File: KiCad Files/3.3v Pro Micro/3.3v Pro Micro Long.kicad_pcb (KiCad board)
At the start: 2 copper layers, 35.7 x 48.3 mm, 5 parts, among them U2 ProMicro, U3 BOB-12009

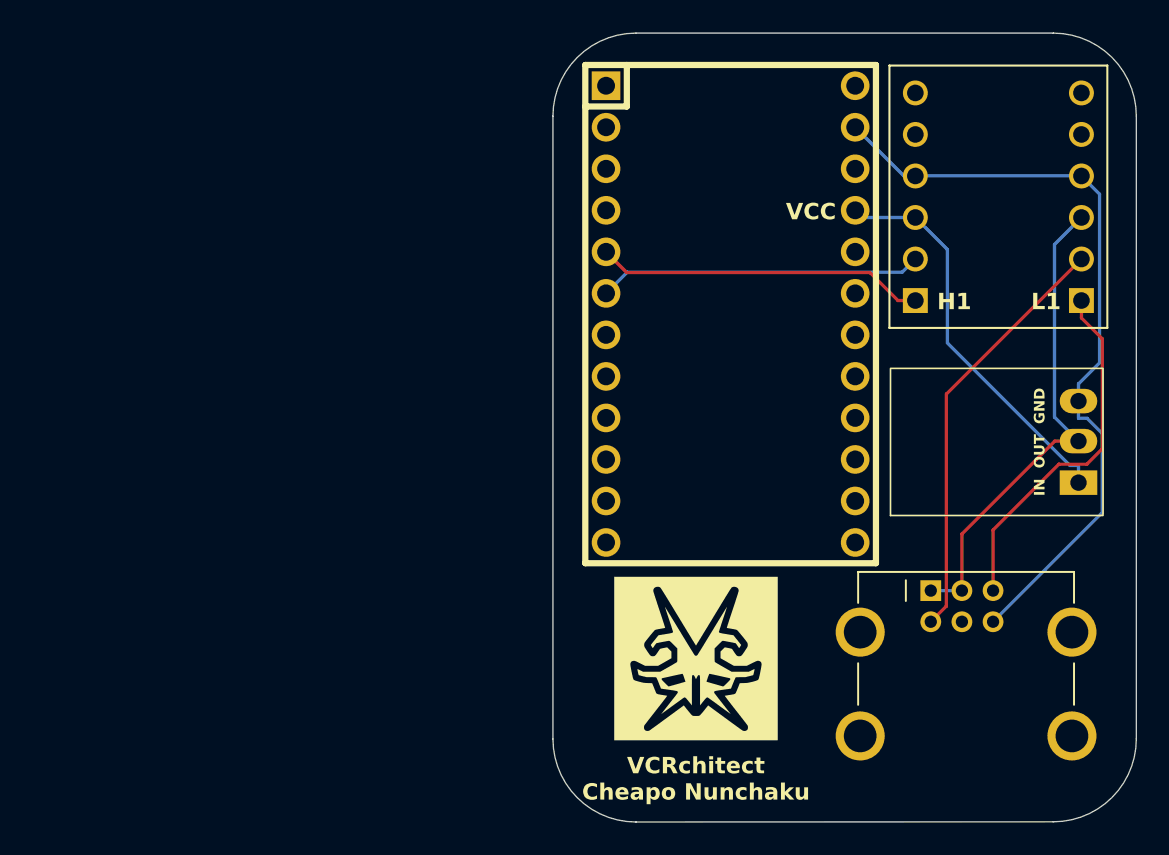
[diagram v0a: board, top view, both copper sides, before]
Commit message: Mini Boss edit
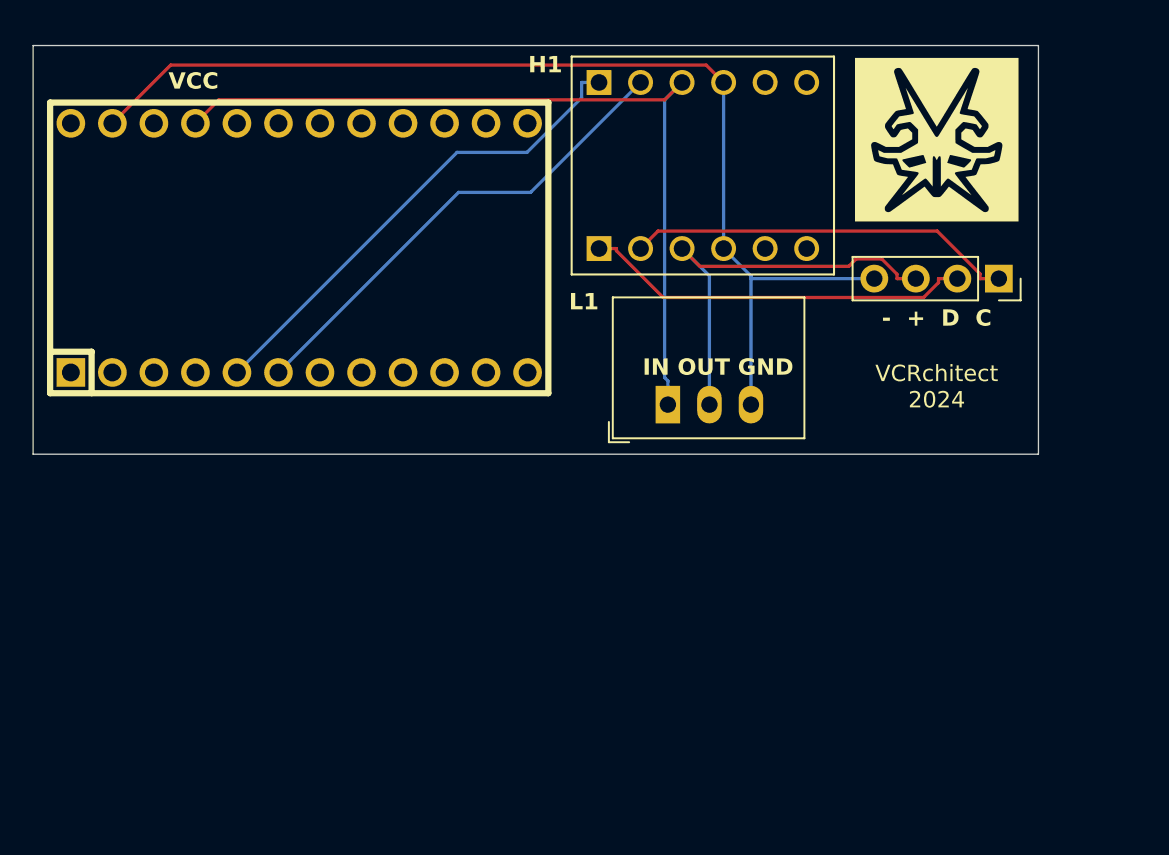
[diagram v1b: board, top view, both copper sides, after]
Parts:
- removed Connector1: Wii Connector, Library:Nintendo_Wii_Peripheral_6Pin_Socket_Horizontal
- added J1: Conn_01x04_Socket, Connector_PinSocket_2.54mm:PinSocket_1x04_P2.54mm_Vertical, F.Cu at (185.3, 93.5)
- U4: footprint Library:3.3v InOutGnd Voltage Regulator -> Converter_DCDC:Converter_DCDC_RECOM_R-78E-0.5_THT
- moved G*** 35.0 mm to (181.5, 85.0)
- moved U4 26.7 mm to (165.1, 101.2), turned to 0 degrees
- moved U2 26.7 mm to (142.5, 91.6), turned to 0 degrees
- moved U3 18.2 mm to (167.2, 86.6), turned to 90 degrees
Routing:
- net Net-(U2-VCC): track 24.5 -> 51.0 mm
- net Net-(J1-Pin_4): track 47.0 -> 67.3 mm
- net Net-(U2-SDA): track 20.2 -> 30.0 mm
- net Net-(U2-SCL): track 19.8 -> 29.5 mm
- net Net-(J1-Pin_3): track 29.8 -> 25.8 mm
- net Net-(J1-Pin_1): track 26.0 -> 23.7 mm
- net Net-(J1-Pin_2): track 22.0 -> 23.9 mm
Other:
- board size 35.7 x 48.3 mm -> 61.5 x 25 mm
- board text added: "- + D C"
- board text added: "IN OUT GND"
- board text added: "VCRchitect 2024"
- board text removed: "VCRchitect Cheapo Nunchaku"
